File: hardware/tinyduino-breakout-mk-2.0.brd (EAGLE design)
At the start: 20 x 20 mm, 5 parts, among them J1 DF12-32-DP

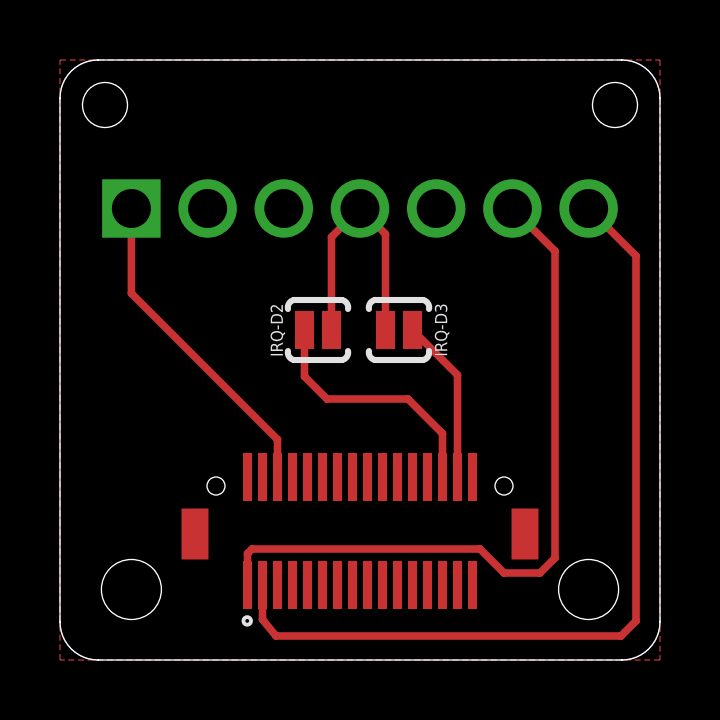
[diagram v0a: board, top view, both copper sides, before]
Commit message: tiny breakout attempt
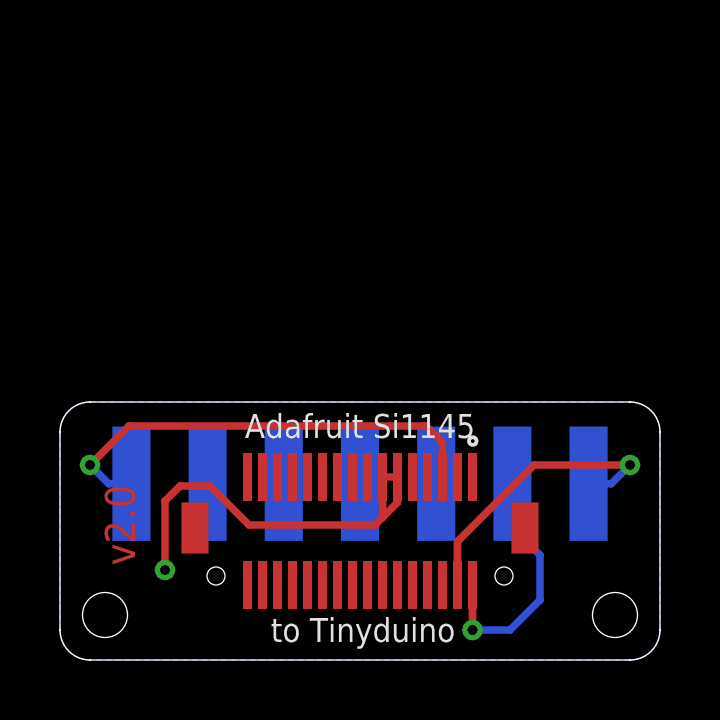
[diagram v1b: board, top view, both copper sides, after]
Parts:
- removed IRQ-D2, IRQ-D3: JUMPER-PAD-2-NOYES_SILK, A_butts:PAD-JUMPER-2-NO_YES_SILK
- BRK1: value ADAFRUIT-SI1145-BREAKOUT -> ADAFRUIT-SI1145-BREAKOUTSMD-RA; device A_butts:ADAFRUIT-SI1145-BREAKOUT -> A_butts:1X07-SMD-SHORT
- J1: value DF12-32-DP -> AS-ITM-00015DF12-32-DP-REV
- moved BRK1 6.00 mm to (10.0, 2.70), turned to 0 degrees
- moved FRAME1 0.50 mm to (0.00, 0.00)
- turned J1 to 180 degrees
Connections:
- removed net D2: IRQ-D2.2, J1.28
- removed net D3: IRQ-D3.2, J1.30
- removed net IRQ: BRK1.IRQ, IRQ-D2.1, IRQ-D3.1
- net GND: now also BRK1.6, J1.11, J1.13; no longer BRK1.GND, J1.12, J1.14
- net SCL: now also BRK1.2, J1.2; no longer BRK1.SCL, J1.1
- net SDA: now also BRK1.1, J1.4; no longer BRK1.SDA, J1.3
- net VCC: now also BRK1.7, J1.5; no longer BRK1.VIN, J1.6
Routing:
- net SDA: track 28.5 -> 9.90 mm, vias 0 -> 1
- net SCL: track 24.1 -> 8.42 mm, vias 0 -> 1
- net GND: track 0.00 -> 13.8 mm, vias 0 -> 1
- net IRQ: track 8.85 -> 0.00 mm
- net D2: track 8.39 -> 0.00 mm
- net D3: track 5.52 -> 0.00 mm
- net VCC: track 11.0 -> 15.3 mm, vias 0 -> 1
- added copper zone on layer 16, net GND
- removed copper zone on layer 1, net GND
- removed copper zone on layer 16, net GND1
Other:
- board size 20 x 20 mm -> 20 x 8.6 mm
- board text added: ">VERSION"
- board text added: "Adafruit Si1145"
- board text added: "to Tinyduino"
- board text removed: "Sensor This Side (face up, in case that wasn't obvious)"
- board text removed: "TinyDuino adapter for Adafruit Si1145 UV i2c Sensor"
